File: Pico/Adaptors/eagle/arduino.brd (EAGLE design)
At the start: 57.1 x 53.3 mm, 5 parts

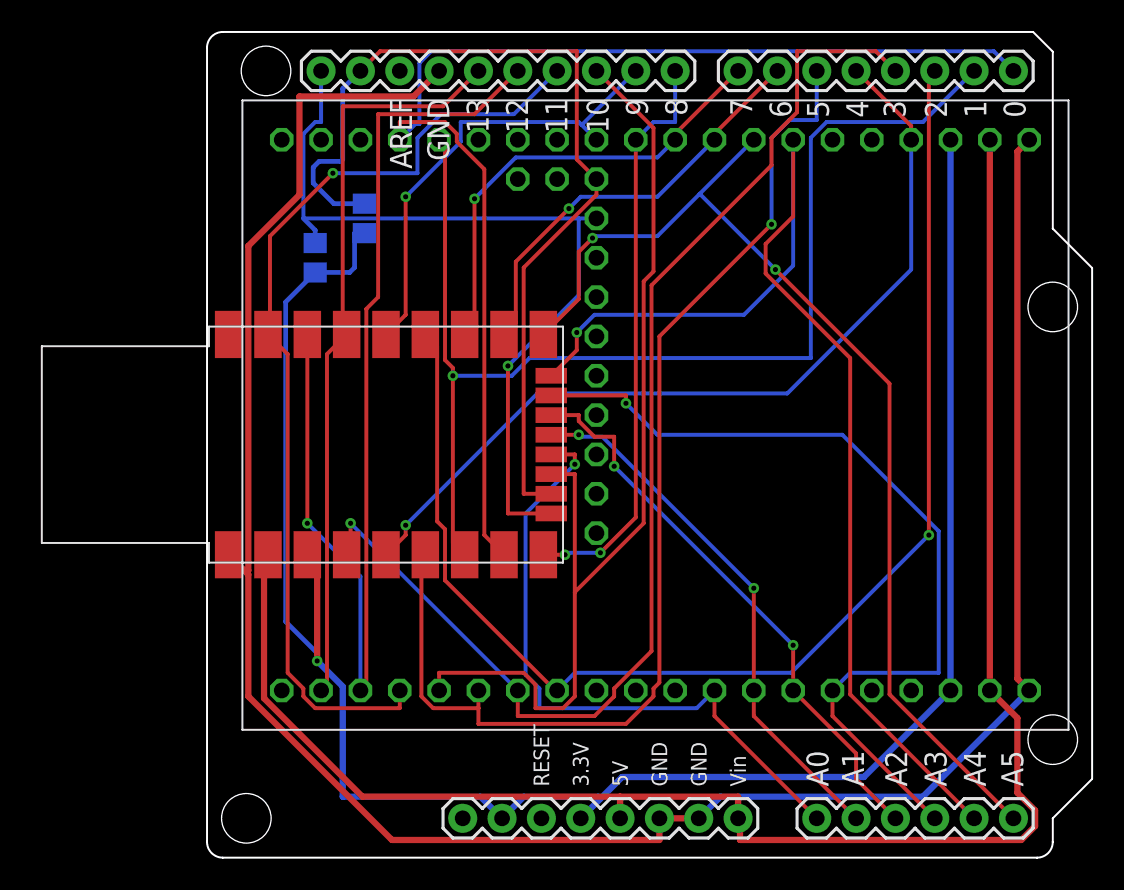
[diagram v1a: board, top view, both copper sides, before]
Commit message: move board around
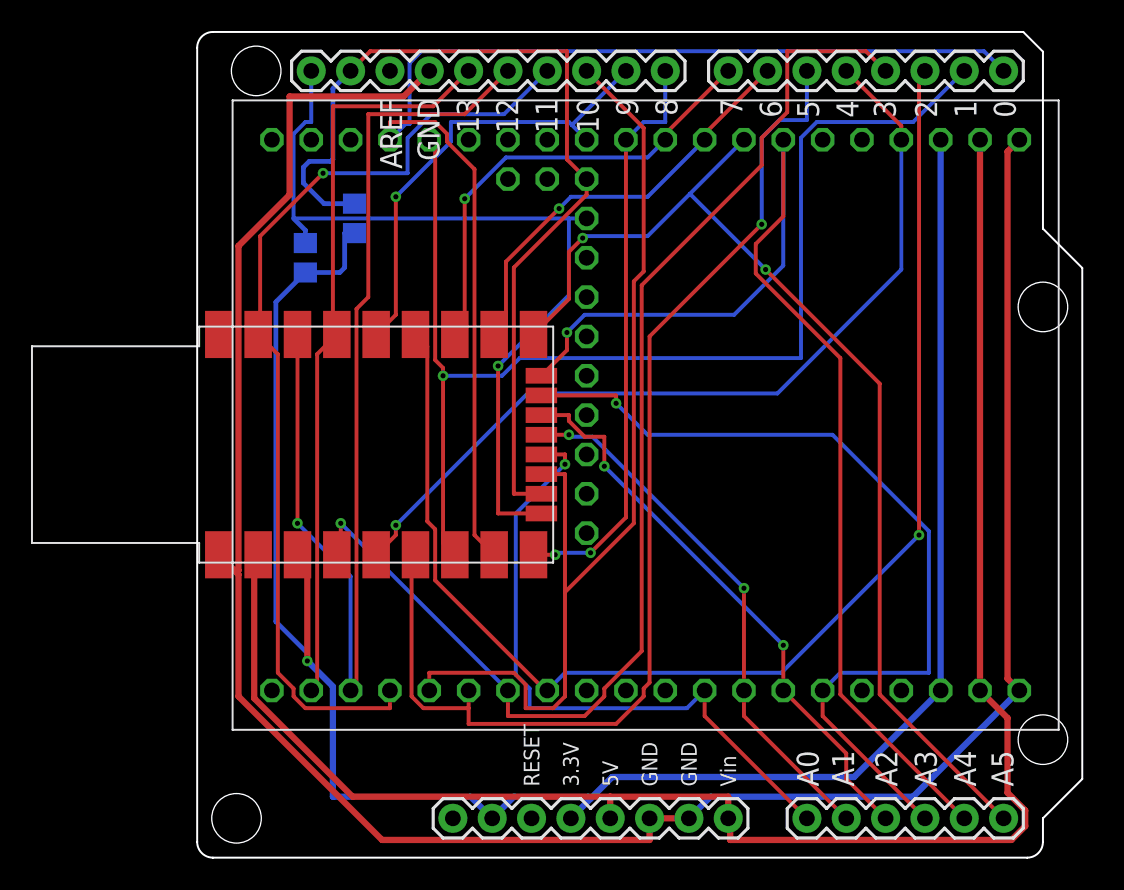
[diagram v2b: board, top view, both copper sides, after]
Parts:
- moved U$2 0.64 mm to (24.1, 26.7)
- moved U$3 0.64 mm to (29.0, 29.8)
- moved R1 0.63 mm to (6.99, 38.7)
- moved R2 0.63 mm to (10.2, 41.3)
- moved U$1 0.63 mm to (15.4, 26.7)

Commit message: a full panel
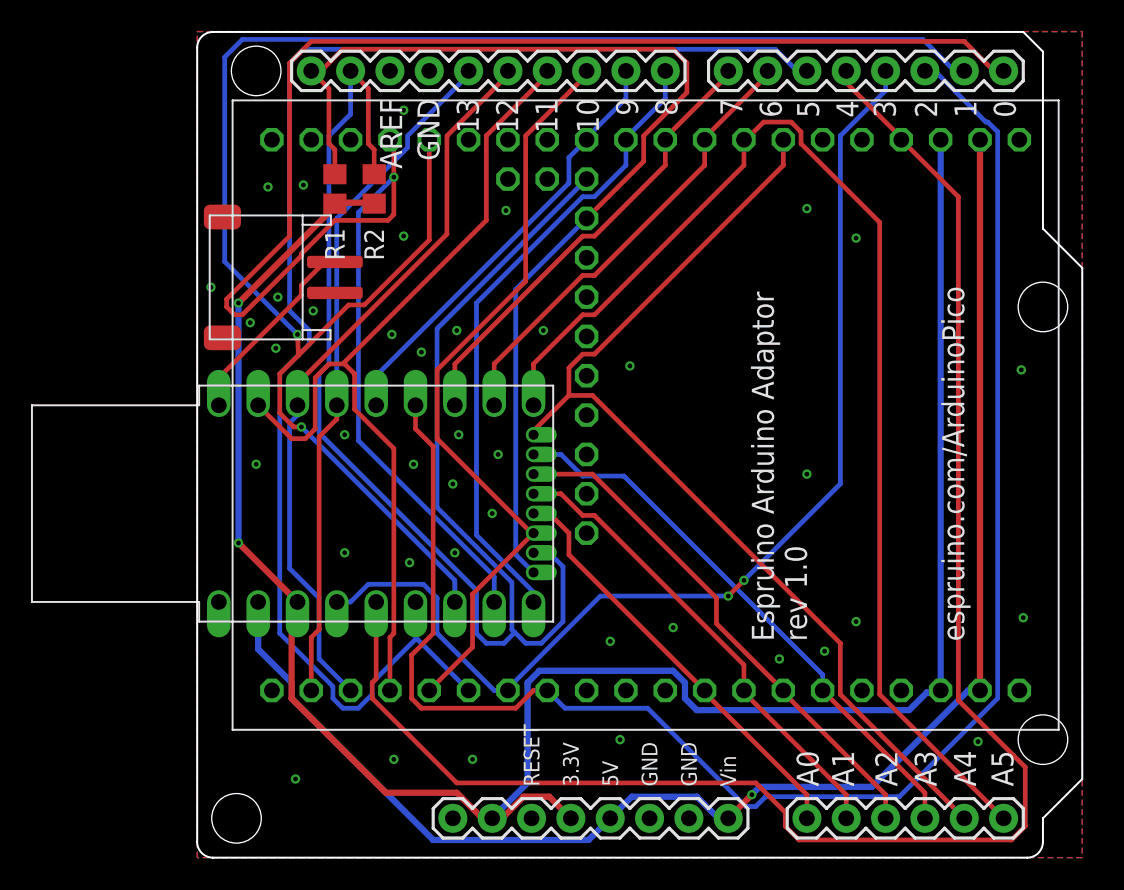
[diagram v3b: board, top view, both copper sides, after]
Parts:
- added J1: JST-2P-SMD-PW-3410050P1, OPL Eagle Library:2P-SMD-2.0-90D
- U$1: value ESPRUINO_PICO_SMDONLY -> ESPRUINO_PICO_SMD; device espruino_pico:ESPRUINO_PICO_SMDONLY -> espruino_pico:ESPRUINO_PICO_SMD
- moved R1 4.84 mm to (8.89, 43.2), flipped to the top
- moved U$1 3.81 mm to (15.4, 22.9)
- moved R2 2.29 mm to (11.4, 43.2), flipped to the top
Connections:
- new net N$1: J1.+, U$1.BAT
- net GND: now also J1.-, J1.3, J1.4
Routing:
- net GND: track 146.8 -> 0.00 mm, vias 0 -> 40
- net D4: track 56.2 -> 106.7 mm, vias 1 -> 0
- net D0: track 78.4 -> 115.6 mm, vias 0 -> 1
- net SDA: track 60.5 -> 96.9 mm
- net D1: track 77.6 -> 109.7 mm, vias 1 -> 2
- net D12: track 72.3 -> 47.5 mm, vias 1 -> 0
- net D2: track 84.9 -> 107.5 mm, vias 1 -> 0
- net D5: track 73.2 -> 93.3 mm, vias 1 -> 0
- net A3: track 56.4 -> 36.6 mm, vias 1 -> 0
- net SCL: track 54.8 -> 70.6 mm, vias 1 -> 0
- net D10: track 65.2 -> 49.4 mm
- net VIN: track 111.8 -> 96.1 mm, vias 0 -> 1
- net A0: track 42.4 -> 27.6 mm, vias 1 -> 0
- net N$1: track 0.00 -> 12.8 mm
- net A4: track 77.5 -> 64.9 mm, vias 1 -> 0
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- added copper zone on layer 1, net GND
- added copper zone on layer 16, net GND
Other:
- board text added: "Espruino Arduino Adaptor rev 1.0"
- board text added: "espruino.com/ArduinoPico"
